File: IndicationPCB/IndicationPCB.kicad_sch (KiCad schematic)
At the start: 0 parts

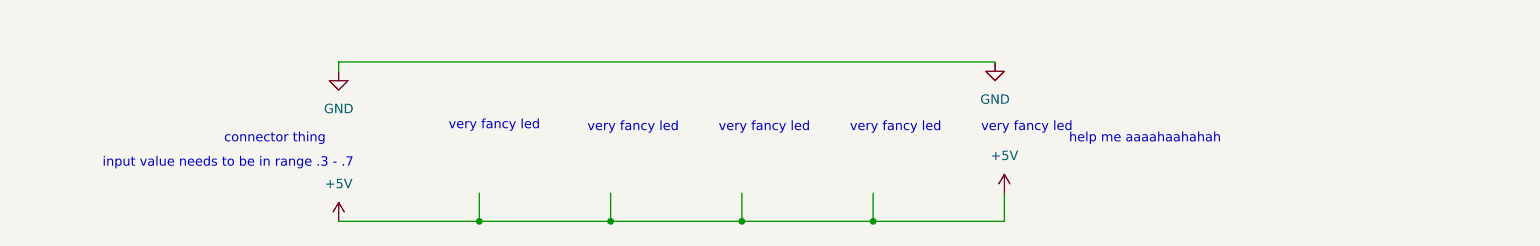
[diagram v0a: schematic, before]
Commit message: Draft
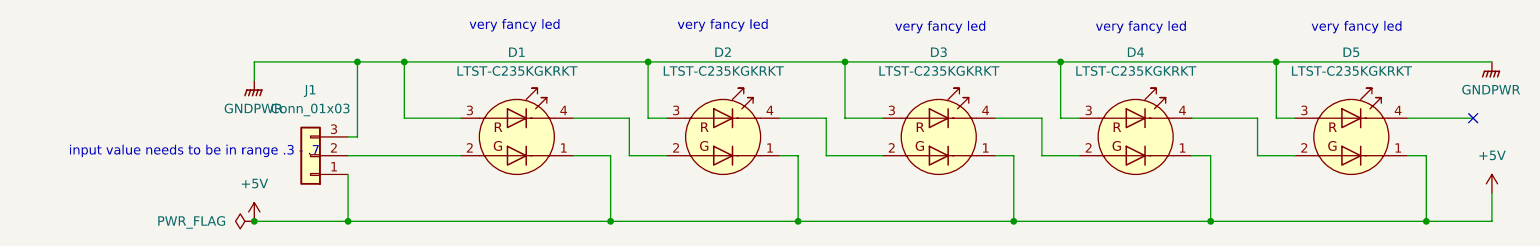
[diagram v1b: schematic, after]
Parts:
- added D1, D2, D3, D4, D5: LTST-C235KGKRKT, LED_SMD:LED_LiteOn_LTST-C235KGKRKT, symbol LED:LTST-C235KGKRKT
- added J1: Conn_01x03, Connector_Molex:Molex_Nano-Fit_105309-xx03_1x03_P2.50mm_Vertical, symbol Connector_Generic:Conn_01x03
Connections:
- net +5V: now also D1.1 (K2), D2.1 (K2), D3.1 (K2), D4.1 (K2), D5.1 (K2), J1.1 (Pin_1)
- new net: D2.4 (K1), D3.2 (A2)
- new net: D3.4 (K1), D4.2 (A2)
- new net: D4.4 (K1), D5.2 (A2)
- new net: D1.4 (K1), D2.2 (A2)
- new net: D1.2 (A2), J1.2 (Pin_2)
- new net GNDPWR: D1.3 (A1), D2.3 (A1), D3.3 (A1), D4.3 (A1), D5.3 (A1), J1.3 (Pin_3)
- no-connect marks 0 -> 1
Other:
- note removed: "connector thing"
- note removed: "help me aaaahaahahah"
